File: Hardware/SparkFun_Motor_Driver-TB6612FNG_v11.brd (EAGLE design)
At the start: 20.3 x 20.3 mm, 14 parts, among them U1 TB6612FNG

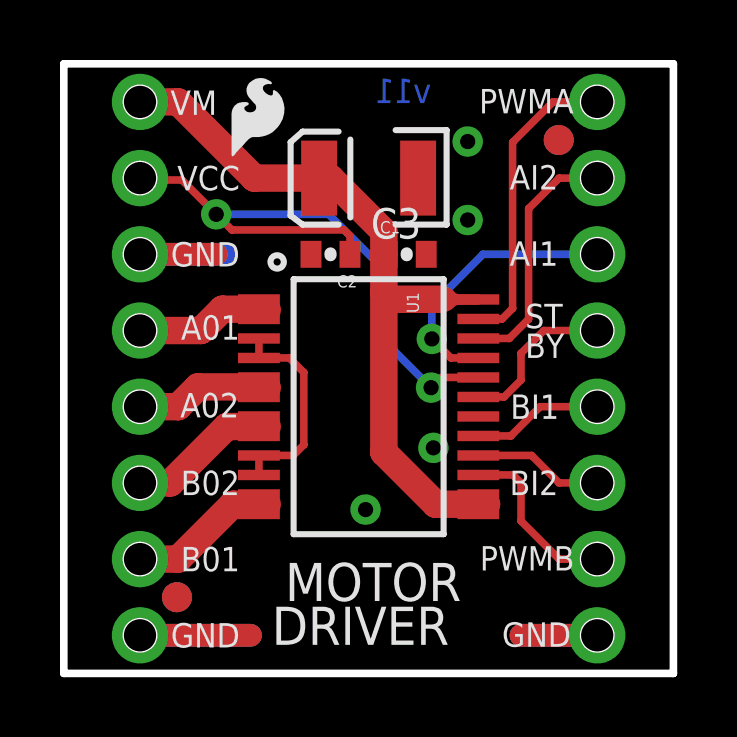
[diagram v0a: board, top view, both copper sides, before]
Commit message: Straightened some silk labels
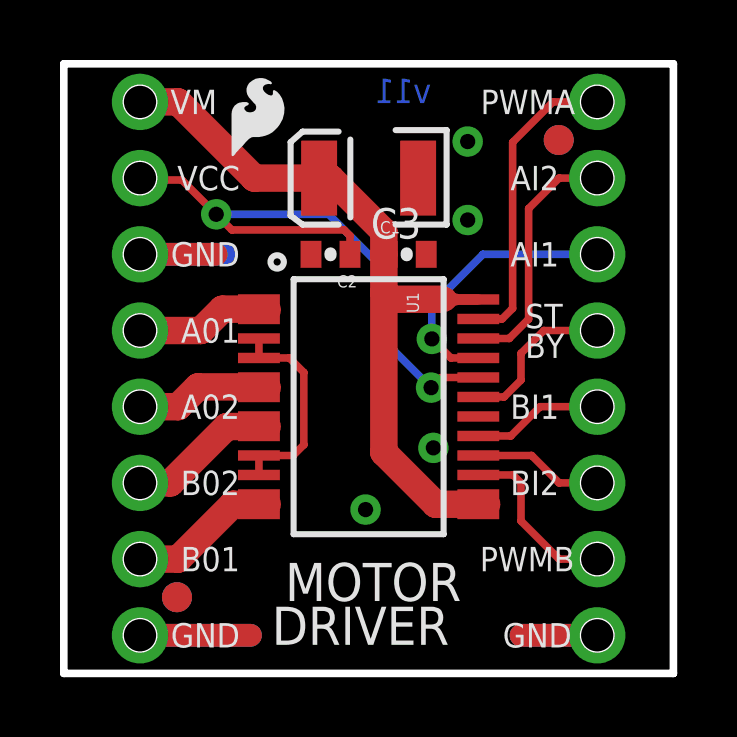
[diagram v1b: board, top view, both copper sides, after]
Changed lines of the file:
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@@
 <setting verticaltext="up"/>
 </settings>
-<grid distance="0.05" unitdist="inch" unit="inch" style="lines" multiple="1" display="yes" altdistance="0.0005" altunitdist="inch" altunit="inch"/>
+<grid distance="0.05" unitdist="inch" unit="inch" style="lines" multiple="1" display="yes" altdistance="0.001" altunitdist="inch" altunit="inch"/>
 <layers>
 <layer number="1" name="Top" color="4" fill="1" visible="yes" active="yes"/>
@@
 <text x="16.51" y="18.542" size="1.016" layer="22" font="vector" ratio="15" rot="MR0">PWMA</text>
 <text x="12.2428" y="19.0119" size="0.8128" layer="16" font="vector" ratio="15" rot="MR0">v11</text>
-<text x="5.1054" y="19.431" size="0.8128" layer="21" font="vector" ratio="15" rot="R180">VM</text>
+<text x="5.1054" y="19.4564" size="0.8128" layer="21" font="vector" ratio="15" rot="R180">VM</text>
 <text x="5.8674" y="16.9164" size="0.8128" layer="21" font="vector" ratio="15" rot="R180">VCC</text>
 <text x="5.8674" y="14.3764" size="0.8128" layer="21" font="vector" ratio="15" rot="R180">GND</text>
 <text x="5.8674" y="1.6764" size="0.8128" layer="21" font="vector" ratio="15" rot="R180">GND</text>
-<text x="14.605" y="0.889" size="0.8128" layer="21" font="vector" ratio="15">GND</text>
-<text x="5.8674" y="11.938" size="0.8128" layer="21" font="vector" ratio="15" rot="R180">A01</text>
-<text x="5.842" y="9.3472" size="0.8128" layer="21" font="vector" ratio="15" rot="R180">A02</text>
+<text x="14.6304" y="0.8636" size="0.8128" layer="21" font="vector" ratio="15">GND</text>
+<text x="5.8674" y="11.8364" size="0.8128" layer="21" font="vector" ratio="15" rot="R180">A01</text>
+<text x="5.8674" y="9.2964" size="0.8128" layer="21" font="vector" ratio="15" rot="R180">A02</text>
 <text x="5.8674" y="6.7564" size="0.8128" layer="21" font="vector" ratio="15" rot="R180">B02</text>
 <text x="5.8674" y="4.2164" size="0.8128" layer="21" font="vector" ratio="15" rot="R180">B01</text>
-<text x="13.8684" y="3.429" size="0.8128" layer="21" font="vector" ratio="15">PWMB</text>
-<text x="14.859" y="5.9436" size="0.8128" layer="21" font="vector" ratio="15">BI2</text>
+<text x="13.8684" y="3.4036" size="0.8128" layer="21" font="vector" ratio="15">PWMB</text>
+<text x="14.8844" y="5.9436" size="0.8128" layer="21" font="vector" ratio="15">BI2</text>
 <text x="14.8844" y="8.4836" size="0.8128" layer="21" font="vector" ratio="15" rot="SR0">BI1</text>
 <text x="15.3797" y="11.5062" size="0.8128" layer="21" font="vector" ratio="15" rot="SR0">ST</text>
-<text x="14.859" y="13.589" size="0.8128" layer="21" font="vector" ratio="15">AI1</text>
-<text x="14.859" y="16.129" size="0.8128" layer="21" font="vector" ratio="15">AI2</text>
-<text x="13.843" y="18.669" size="0.8128" layer="21" font="vector" ratio="15">PWMA</text>
+<text x="14.8844" y="13.5636" size="0.8128" layer="21" font="vector" ratio="15">AI1</text>
+<text x="14.8844" y="16.1036" size="0.8128" layer="21" font="vector" ratio="15">AI2</text>
+<text x="13.8938" y="18.6436" size="0.8128" layer="21" font="vector" ratio="15">PWMA</text>
 <text x="15.3797" y="10.5156" size="0.8128" layer="21" font="vector" ratio="15" rot="SR0">BY</text>
 <text x="7.3787" y="2.413" size="1.27" layer="21" font="vector" ratio="15">MOTOR</text>
